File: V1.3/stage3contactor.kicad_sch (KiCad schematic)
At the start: 9 parts, among them J10 Screw_Terminal_01x02, J11 Screw_Terminal_01x02, J12 Screw_Terminal_01x02, J14 Screw_Terminal_01x02, J5 Screw_Terminal_01x02, J6 Screw_Terminal_01x02, J7 Screw_Terminal_01x02, J8 Screw_Terminal_01x02, J9 Screw_Terminal_01x02

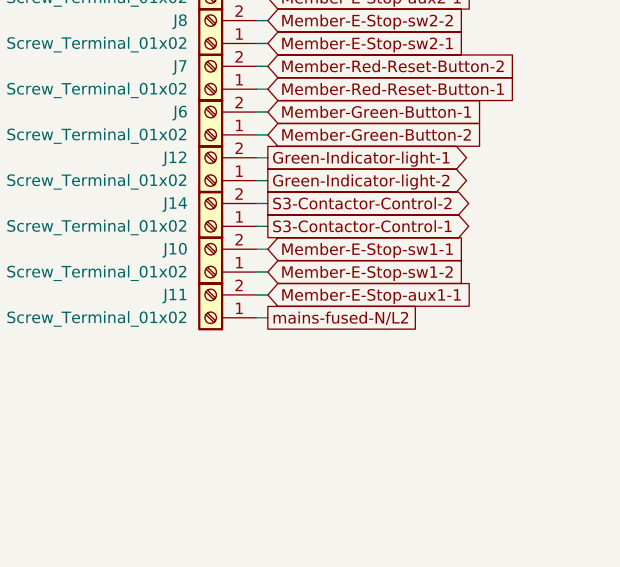
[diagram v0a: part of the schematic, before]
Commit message: fixing edges and connecting all pieces
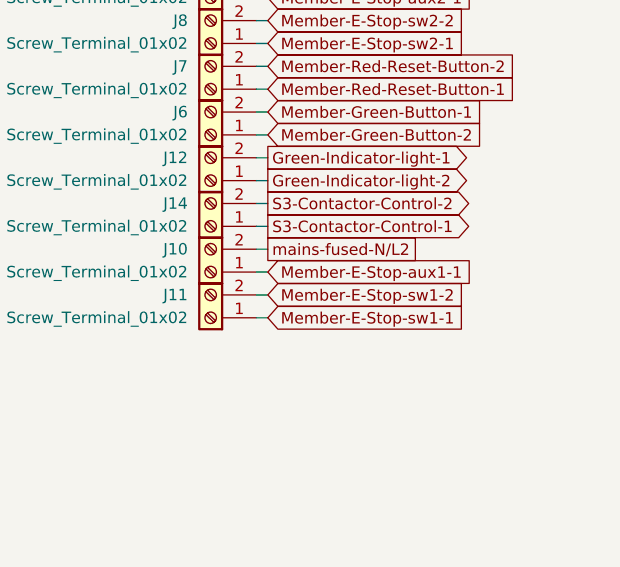
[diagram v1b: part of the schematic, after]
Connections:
- net Member-E-Stop-sw1-1: now also J11.1 (Pin_1); no longer J10.2 (Pin_2)
- net mains-fused-N/L2: now also J10.2 (Pin_2); no longer J11.1 (Pin_1)
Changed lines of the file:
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@@
   (junction (at 66.04 105.41) (diameter 0) (color 0 0 0 0)
   )
+  (wire (pts (xy 201.93 134.62) (xy 203.2 134.62))
+    (stroke (width 0) (type default) (color 0 0 0 0))
+  )
   (wire (pts (xy 66.04 101.6) (xy 66.04 105.41))
     (stroke (width 0) (type default) (color 0 0 0 0))
@@
     (stroke (width 0) (type default) (color 0 0 0 0))
   )
-  (wire (pts (xy 201.93 134.62) (xy 203.2 134.62))
-    (stroke (width 0) (type default) (color 0 0 0 0))
-  )
   (wire (pts (xy 66.04 105.41) (xy 66.04 115.57))
     (stroke (width 0) (type default) (color 0 0 0 0))
   )
+  (wire (pts (xy 66.04 95.25) (xy 100.33 95.25))
+    (stroke (width 0) (type default) (color 0 0 0 0))
+  )
+  (wire (pts (xy 66.04 130.81) (xy 66.04 152.4))
+    (stroke (width 0) (type default) (color 0 0 0 0))
+  )
+  (wire (pts (xy 201.93 127) (xy 203.2 127))
+    (stroke (width 0) (type default) (color 0 0 0 0))
+  )
+  (wire (pts (xy 201.93 96.52) (xy 203.2 96.52))
+    (stroke (width 0) (type default) (color 0 0 0 0))
+  )
+  (wire (pts (xy 201.93 109.22) (xy 203.2 109.22))
+    (stroke (width 0) (type default) (color 0 0 0 0))
+  )
+  (wire (pts (xy 66.04 105.41) (xy 100.33 105.41))
+    (stroke (width 0) (type default) (color 0 0 0 0))
+  )
+  (wire (pts (xy 201.93 114.3) (xy 203.2 114.3))
+    (stroke (width 0) (type default) (color 0 0 0 0))
+  )
+  (wire (pts (xy 201.93 93.98) (xy 203.2 93.98))
+    (stroke (width 0) (type default) (color 0 0 0 0))
+  )
+  (wire (pts (xy 66.04 95.25) (xy 66.04 99.06))
+    (stroke (width 0) (type default) (color 0 0 0 0))
+  )
+  (polyline (pts (xy 64.77 132.08) (xy 64.77 127))
+    (stroke (width 0) (type default) (color 0 0 0 0))
+  )
+  (wire (pts (xy 201.93 121.92) (xy 203.2 121.92))
+    (stroke (width 0) (type default) (color 0 0 0 0))
+  )
+  (polyline (pts (xy 64.77 151.13) (xy 64.77 156.21))
+    (stroke (width 0) (type default) (color 0 0 0 0))
+  )
+  (wire (pts (xy 66.04 119.38) (xy 66.04 128.27))
+    (stroke (width 0) (type default) (color 0 0 0 0))
+  )
+  (wire (pts (xy 201.93 104.14) (xy 203.2 104.14))
+    (stroke (width 0) (type default) (color 0 0 0 0))
+  )
+  (wire (pts (xy 201.93 101.6) (xy 203.2 101.6))
+    (stroke (width 0) (type default) (color 0 0 0 0))
+  )
+  (wire (pts (xy 66.04 90.17) (xy 66.04 95.25))
+    (stroke (width 0) (type default) (color 0 0 0 0))
+  )
+  (wire (pts (xy 201.93 99.06) (xy 203.2 99.06))
+    (stroke (width 0) (type default) (color 0 0 0 0))
+  )
+  (wire (pts (xy 201.93 132.08) (xy 203.2 132.08))
+    (stroke (width 0) (type default) (color 0 0 0 0))
+  )
+  (wire (pts (xy 201.93 106.68) (xy 203.2 106.68))
+    (stroke (width 0) (type default) (color 0 0 0 0))
+  )
   (wire (pts (xy 201.93 137.16) (xy 203.2 137.16))
     (stroke (width 0) (type default) (color 0 0 0 0))
   )
-  (wire (pts (xy 66.04 95.25) (xy 100.33 95.25))
-    (stroke (width 0) (type default) (color 0 0 0 0))
-  )
-  (wire (pts (xy 66.04 130.81) (xy 66.04 152.4))
-    (stroke (width 0) (type default) (color 0 0 0 0))
-  )
-  (wire (pts (xy 201.93 127) (xy 203.2 127))
-    (stroke (width 0) (type default) (color 0 0 0 0))
-  )
-  (wire (pts (xy 201.93 96.52) (xy 203.2 96.52))
-    (stroke (width 0) (type default) (color 0 0 0 0))
-  )
-  (wire (pts (xy 201.93 109.22) (xy 203.2 109.22))
-    (stroke (width 0) (type default) (color 0 0 0 0))
-  )
-  (wire (pts (xy 66.04 105.41) (xy 100.33 105.41))
-    (stroke (width 0) (type default) (color 0 0 0 0))
-  )
-  (wire (pts (xy 201.93 114.3) (xy 203.2 114.3))
-    (stroke (width 0) (type default) (color 0 0 0 0))
-  )
-  (wire (pts (xy 201.93 93.98) (xy 203.2 93.98))
-    (stroke (width 0) (type default) (color 0 0 0 0))
-  )
-  (wire (pts (xy 66.04 95.25) (xy 66.04 99.06))
-    (stroke (width 0) (type default) (color 0 0 0 0))
-  )
-  (wire (pts (xy 201.93 132.08) (xy 203.2 132.08))
-    (stroke (width 0) (type default) (color 0 0 0 0))
-  )
-  (polyline (pts (xy 64.77 132.08) (xy 64.77 127))
-    (stroke (width 0) (type default) (color 0 0 0 0))
-  )
-  (wire (pts (xy 201.93 121.92) (xy 203.2 121.92))
-    (stroke (width 0) (type default) (color 0 0 0 0))
-  )
-  (polyline (pts (xy 64.77 151.13) (xy 64.77 156.21))
-    (stroke (width 0) (type default) (color 0 0 0 0))
-  )
-  (wire (pts (xy 66.04 119.38) (xy 66.04 128.27))
-    (stroke (width 0) (type default) (color 0 0 0 0))
-  )
-  (wire (pts (xy 201.93 104.14) (xy 203.2 104.14))
-    (stroke (width 0) (type default) (color 0 0 0 0))
-  )
-  (wire (pts (xy 201.93 101.6) (xy 203.2 101.6))
-    (stroke (width 0) (type default) (color 0 0 0 0))
-  )
-  (wire (pts (xy 66.04 90.17) (xy 66.04 95.25))
-    (stroke (width 0) (type default) (color 0 0 0 0))
-  )
-  (wire (pts (xy 201.93 99.06) (xy 203.2 99.06))
-    (stroke (width 0) (type default) (color 0 0 0 0))
-  )
-  (wire (pts (xy 201.93 106.68) (xy 203.2 106.68))
+  (wire (pts (xy 201.93 119.38) (xy 203.2 119.38))
+    (stroke (width 0) (type default) (color 0 0 0 0))
+  )
+  (wire (pts (xy 201.93 124.46) (xy 203.2 124.46))
+    (stroke (width 0) (type default) (color 0 0 0 0))
+  )
+  (wire (pts (xy 201.93 116.84) (xy 203.2 116.84))
     (stroke (width 0) (type default) (color 0 0 0 0))
   )
   (wire (pts (xy 201.93 129.54) (xy 203.2 129.54))
-    (stroke (width 0) (type default) (color 0 0 0 0))
-  )
-  (wire (pts (xy 201.93 119.38) (xy 203.2 119.38))
-    (stroke (width 0) (type default) (color 0 0 0 0))
-  )
-  (wire (pts (xy 201.93 124.46) (xy 203.2 124.46))
-    (stroke (width 0) (type default) (color 0 0 0 0))
-  )
-  (wire (pts (xy 201.93 116.84) (xy 203.2 116.84))
     (stroke (width 0) (type default) (color 0 0 0 0))
   )
@@
     )
   )
-  (global_label "mains-fused-N{slash}L2" (shape passive) (at 203.2 137.16 0) (fields_autoplaced)
-    (effects (font (size 1.27 1.27)) (justify left))
-    (property "Intersheet References" "${INTERSHEET_REFS}" (id 0) (at 224.4212 137.0806 0)
+  (global_label "mains-fused-N{slash}L2" (shape passive) (at 203.2 129.54 0) (fields_autoplaced)
+    (effects (font (size 1.27 1.27)) (justify left))
+    (property "Intersheet References" "${INTERSHEET_REFS}" (id 0) (at 224.4212 129.4606 0)
       (effects (font (size 1.27 1.27)) (justify left) hide)
     )
@@
     )
   )
-  (global_label "Member-E-Stop-sw1-2" (shape input) (at 203.2 132.08 0) (fields_autoplaced)
-    (effects (font (size 1.27 1.27)) (justify left))
-    (property "Intersheet References" "${INTERSHEET_REFS}" (id 0) (at 229.3198 132.0006 0)
+  (global_label "Member-E-Stop-sw1-2" (shape input) (at 203.2 134.62 0) (fields_autoplaced)
+    (effects (font (size 1.27 1.27)) (justify left))
+    (property "Intersheet References" "${INTERSHEET_REFS}" (id 0) (at 229.3198 134.5406 0)
       (effects (font (size 1.27 1.27)) (justify left) hide)
     )
@@
     )
   )
-  (global_label "Member-E-Stop-aux1-1" (shape input) (at 203.2 134.62 0) (fields_autoplaced)
-    (effects (font (size 1.27 1.27)) (justify left))
-    (property "Intersheet References" "${INTERSHEET_REFS}" (id 0) (at 230.2874 134.5406 0)
+  (global_label "Member-E-Stop-aux1-1" (shape input) (at 203.2 132.08 0) (fields_autoplaced)
+    (effects (font (size 1.27 1.27)) (justify left))
+    (property "Intersheet References" "${INTERSHEET_REFS}" (id 0) (at 230.2874 132.0006 0)
       (effects (font (size 1.27 1.27)) (justify left) hide)
     )
@@
     )
   )
-  (global_label "Member-E-Stop-sw1-1" (shape input) (at 203.2 129.54 0) (fields_autoplaced)
-    (effects (font (size 1.27 1.27)) (justify left))
-    (property "Intersheet References" "${INTERSHEET_REFS}" (id 0) (at 229.3198 129.4606 0)
-      (effects (font (size 1.27 1.27)) (justify left) hide)
-    )
+  (global_label "Member-E-Stop-sw1-1" (shape input) (at 203.2 137.16 0) (fields_autoplaced)
+    (effects (font (size 1.27 1.27)) (justify left))
+    (property "Intersheet References" "${INTERSHEET_REFS}" (id 0) (at 229.3198 137.0806 0)
+      (effects (font (size 1.27 1.27)) (justify left) hide)
+    )
